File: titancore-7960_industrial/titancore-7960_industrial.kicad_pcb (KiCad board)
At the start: 2 copper layers, 50.3 x 45 mm, 34 parts, among them J1 XT30, J2 Pin Header M 01x08, J3 XT30, J4 XT30, Q1 BTN8982TA, Q2 BTN8982TA, Q3 BTN8982TA, Q4 BTN8982TA, U5 74HC244

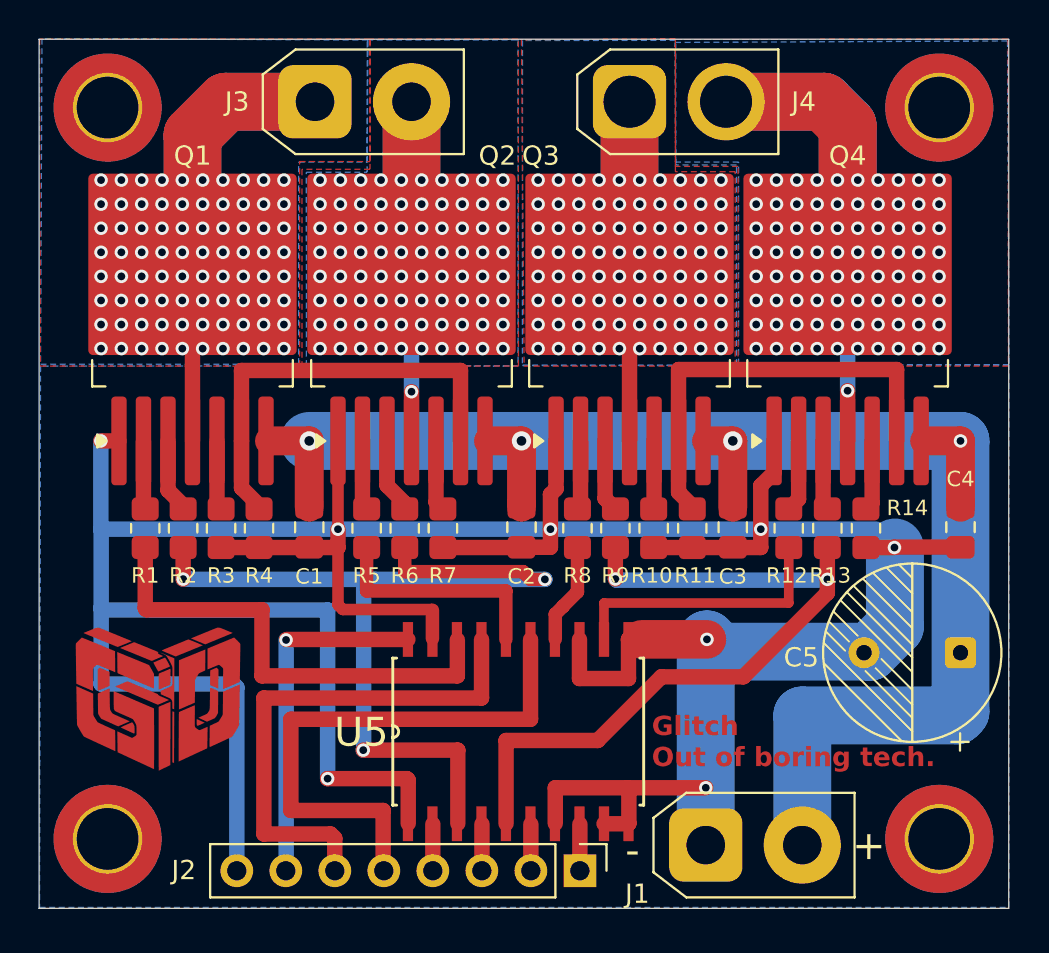
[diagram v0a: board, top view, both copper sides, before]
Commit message: + profesional
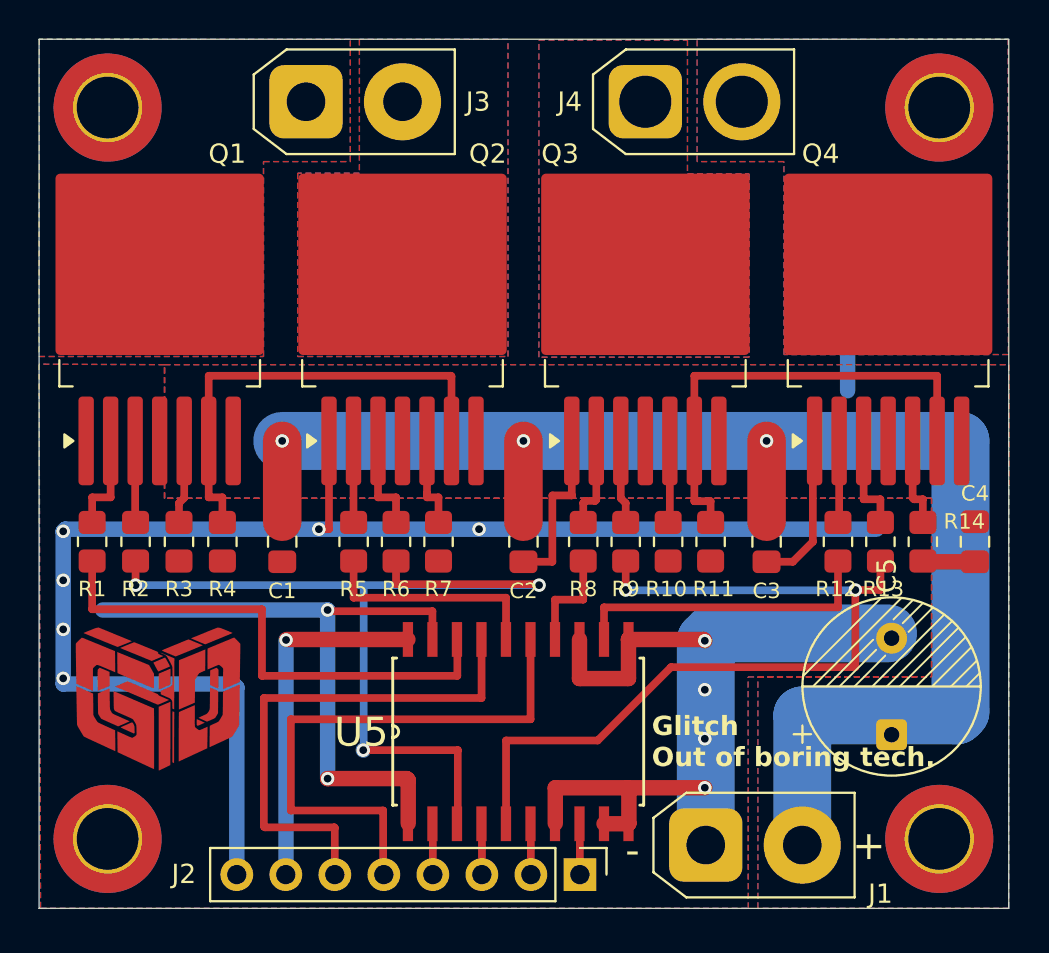
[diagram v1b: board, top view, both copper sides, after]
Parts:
- moved C5 5.55 mm to (153.2, 70.8), turned to 90 degrees
- moved R14 3.03 mm to (154.8, 60.8)
- moved R1 2.84 mm to (111.8, 60.8)
- moved R13 2.84 mm to (152.7, 60.8)
- moved R12 2.64 mm to (150.4, 60.8)
- moved R2 2.56 mm to (114.0, 60.8)
- moved R3 2.29 mm to (116.3, 60.8)
- moved Q4 2.10 mm to (153.1, 47.9)
- moved R4 2.02 mm to (118.5, 60.8)
- moved C3 1.90 mm to (146.8, 60.8)
- moved Q1 1.70 mm to (115.3, 47.9)
- moved C1 1.59 mm to (121.7, 60.8)
- moved R11 1.18 mm to (143.8, 60.8)
- moved C4 1.06 mm to (157.6, 60.8)
- moved R10 1.03 mm to (141.7, 60.8)
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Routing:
- net Net-(J3-Pin_1): track 37.5 -> 0.00 mm, vias 80 -> 0
- net Net-(J4-Pin_2): track 37.4 -> 9.52 mm, vias 81 -> 0
- net GND: track 196.2 -> 171.0 mm, vias 8 -> 12
- net Net-(J4-Pin_1): track 26.0 -> 0.92 mm, vias 80 -> 0
- net Net-(J3-Pin_2): track 26.0 -> 1.13 mm, vias 81 -> 0
- net VS: track 83.5 -> 76.7 mm, vias 4 -> 3
- net OUT_EN_2: track 39.1 -> 44.2 mm
- net OUT_A: track 24.6 -> 26.7 mm
- net Net-(Q3-IS): track 22.5 -> 24.4 mm
- net OUT_D: track 14.3 -> 16.1 mm
- net Net-(Q1-IS): track 22.6 -> 24.2 mm
- net Net-(Q1-IN): track 3.56 -> 5.19 mm
- net Net-(Q4-INH): track 3.62 -> 5.00 mm
- net Net-(Q2-INH): track 3.91 -> 5.16 mm
- net Net-(Q3-IN): track 3.59 -> 4.80 mm
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- added copper zone on F.Cu, net GND
- added copper zone on B.Cu, net VS
- added copper zone on F.Cu, net VS
